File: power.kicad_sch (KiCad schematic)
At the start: 27 parts, among them IC1 SiC437BED-T1-GE3, J4 Barrel_Jack_Switch, Q1 PXP012-30QLJ, Q2 PXP012-30QLJ, U2 LTC4412xS6

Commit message: update 2 everything is fixed
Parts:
- R4, R5: footprint Resistor_SMD:R_2010_5025Metric_Pad1.40x2.65mm_HandSolder -> Resistor_SMD:R_0402_1005Metric
- R6: footprint Resistor_SMD:R_0603_1608Metric_Pad0.98x0.95mm_HandSolder -> Resistor_SMD:R_0402_1005Metric
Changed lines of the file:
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@@
 			)
 		)
-		(property "Footprint" "Resistor_SMD:R_0603_1608Metric_Pad0.98x0.95mm_HandSolder"
+		(property "Footprint" "Resistor_SMD:R_0402_1005Metric"
 			(at 234.95 59.69 0)
 			(effects
@@
 			)
 		)
-		(property "Footprint" "Resistor_SMD:R_2010_5025Metric_Pad1.40x2.65mm_HandSolder"
+		(property "Footprint" "Resistor_SMD:R_0402_1005Metric"
 			(at 201.93 50.8 0)
 			(effects
@@
 			)
 		)
-		(property "Footprint" "Resistor_SMD:R_2010_5025Metric_Pad1.40x2.65mm_HandSolder"
+		(property "Footprint" "Resistor_SMD:R_0402_1005Metric"
 			(at 201.93 48.26 0)
 			(effects

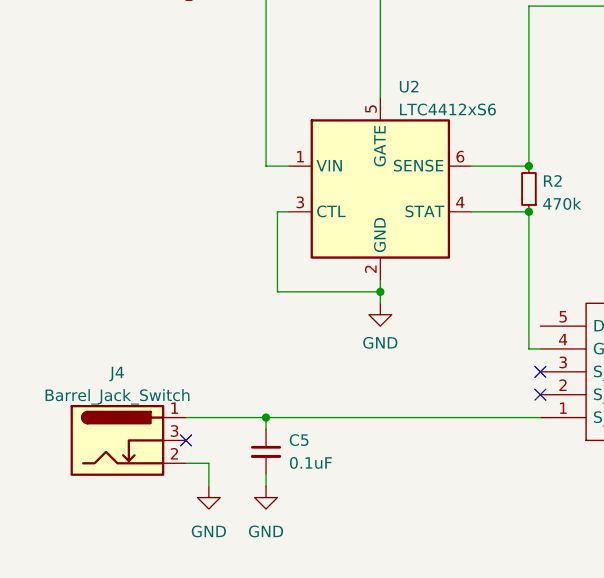
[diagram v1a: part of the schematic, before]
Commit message: ideal diode update to be checked
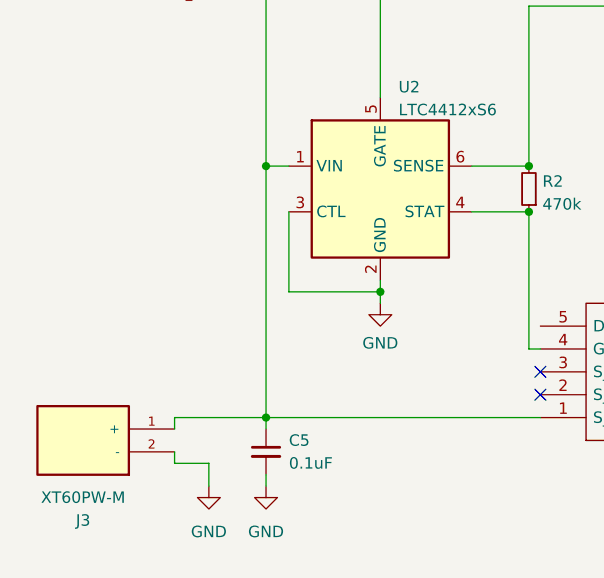
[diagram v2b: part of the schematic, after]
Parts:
- removed J4: Barrel_Jack_Switch, Connector_BarrelJack:BarrelJack_Wuerth_6941xx301002, symbol Connector:Barrel_Jack_Switch
- added J3: XT60PW-M, iclr:AMASS_XT60PW-M, symbol ICLR:XT60PW-M
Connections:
- net +BATTV: now also C5.1, Q2.1 (S_1), J3.1 (+)
- net GND: now also J3.2 (-)
- no-connect marks 17 -> 16
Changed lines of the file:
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@@
 	)
 	(junction
+		(at 44.45 58.42)
+		(diameter 0)
+		(color 0 0 0 0)
+	)
+	(junction
 		(at 196.85 90.17)
 		(diameter 0)
@@
 	)
 	(no_connect
-		(at 35.56 88.9)
-	)
-	(no_connect
 		(at 156.21 60.96)
 	)
@@
 	(wire
 		(pts
+			(xy 44.45 58.42) (xy 44.45 86.36)
+		)
+		(stroke
+			(width 0)
+			(type default)
+		)
+	)
+	(wire
+		(pts
 			(xy 67.31 63.5) (xy 73.66 63.5)
 		)
@@
 	(wire
 		(pts
-			(xy 57.15 71.12) (xy 57.15 72.39)
+			(xy 34.29 87.63) (xy 34.29 86.36)
 		)
 		(stroke
@@
 	(wire
 		(pts
-			(xy 191.77 66.04) (xy 194.31 66.04)
+			(xy 57.15 71.12) (xy 57.15 72.39)
 		)
 		(stroke
@@
 	(wire
 		(pts
-			(xy 217.17 85.09) (xy 217.17 83.82)
+			(xy 191.77 66.04) (xy 194.31 66.04)
 		)
 		(stroke
@@
 	(wire
 		(pts
-			(xy 46.99 63.5) (xy 45.72 63.5)
+			(xy 34.29 90.17) (xy 34.29 91.44)
 		)
 		(stroke
@@
 	(wire
 		(pts
-			(xy 101.6 81.28) (xy 101.6 62.23)
+			(xy 217.17 85.09) (xy 217.17 83.82)
 		)
 		(stroke
@@
 	(wire
 		(pts
-			(xy 148.59 50.8) (xy 148.59 53.34)
+			(xy 101.6 81.28) (xy 101.6 62.23)
 		)
 		(stroke
@@
 	(wire
 		(pts
-			(xy 35.56 91.44) (xy 38.1 91.44)
+			(xy 148.59 50.8) (xy 148.59 53.34)
 		)
 		(stroke
@@
 	(wire
 		(pts
-			(xy 45.72 63.5) (xy 45.72 72.39)
+			(xy 46.99 63.5) (xy 46.99 72.39)
 		)
 		(stroke
@@
 	(wire
 		(pts
-			(xy 44.45 58.42) (xy 46.99 58.42)
+			(xy 187.96 83.82) (xy 196.85 83.82)
 		)
 		(stroke
@@
 	(wire
 		(pts
-			(xy 187.96 83.82) (xy 196.85 83.82)
+			(xy 241.3 68.58) (xy 241.3 59.69)
 		)
 		(stroke
@@
 	(wire
 		(pts
-			(xy 241.3 68.58) (xy 241.3 59.69)
+			(xy 185.42 90.17) (xy 196.85 90.17)
 		)
 		(stroke
@@
 	(wire
 		(pts
-			(xy 185.42 90.17) (xy 196.85 90.17)
+			(xy 147.32 35.56) (xy 147.32 38.1)
 		)
 		(stroke
@@
 	(wire
 		(pts
-			(xy 147.32 35.56) (xy 147.32 38.1)
+			(xy 143.51 63.5) (xy 143.51 73.66)
 		)
 		(stroke
@@
 	(wire
 		(pts
-			(xy 143.51 63.5) (xy 143.51 73.66)
+			(xy 67.31 58.42) (xy 73.66 58.42)
 		)
 		(stroke
@@
 	(wire
 		(pts
-			(xy 67.31 58.42) (xy 73.66 58.42)
+			(xy 34.29 86.36) (xy 44.45 86.36)
 		)
 		(stroke
@@
 	(wire
 		(pts
+			(xy 44.45 58.42) (xy 46.99 58.42)
+		)
+		(stroke
+			(width 0)
+			(type default)
+		)
+	)
+	(wire
+		(pts
 			(xy 87.63 40.64) (xy 101.6 40.64)
 		)
@@
 	(wire
 		(pts
-			(xy 45.72 72.39) (xy 57.15 72.39)
+			(xy 46.99 72.39) (xy 57.15 72.39)
 		)
 		(stroke
@@
 	(wire
 		(pts
-			(xy 35.56 86.36) (xy 44.45 86.36)
-		)
-		(stroke
-			(width 0)
-			(type default)
-		)
-	)
-	(wire
-		(pts
 			(xy 143.51 45.72) (xy 143.51 63.5)
 		)
@@
 	(wire
 		(pts
+			(xy 34.29 91.44) (xy 38.1 91.44)
+		)
+		(stroke
+			(width 0)
+			(type default)
+		)
+	)
+	(wire
+		(pts
 			(xy 132.08 50.8) (xy 132.08 38.1)
 		)
@@
 	)
 	(symbol
-		(lib_id "Connector:Barrel_Jack_Switch")
-		(at 27.94 88.9 0)
-		(unit 1)
-		(exclude_from_sim no)
-		(in_bom yes)
-		(on_board yes)
-		(dnp no)
-		(property "Reference" "J4"
-			(at 27.94 81.3902 0)
-			(effects
-				(font
-					(size 1.27 1.27)
-				)
-			)
-		)
-		(property "Value" "Barrel_Jack_Switch"
-			(at 27.94 83.9271 0)
-			(effects
-				(font
-					(size 1.27 1.27)
-				)
-			)
-		)
-		(property "Footprint" "Connector_BarrelJack:BarrelJack_Wuerth_6941xx301002"
-			(at 29.21 89.916 0)
-			(effects
-				(font
-					(size 1.27 1.27)
-				)
-				(hide yes)
-			)
-		)
-		(property "Datasheet" "~"
-			(at 29.21 89.916 0)
-			(effects
-				(font
-					(size 1.27 1.27)
-				)
-				(hide yes)
-			)
-		)
-		(property "Description" ""
-			(at 27.94 88.9 0)
-			(effects
-				(font
-					(size 1.27 1.27)
-				)
-				(hide yes)
-			)
-		)
-		(pin "1"
-		)
-		(pin "2"
-		)
-		(pin "3"
-		)
-		(instances
-			(project "BetetrDom"
-				(path "/3d73b00f-865e-402b-88ef-ae22e0a8ba36/837d0d5a-cb41-4001-b9fc-855d4a9018ff"
-					(reference "J4")
-					(unit 1)
-				)
-			)
-		)
-	)
-	(symbol
 		(lib_id "power:VCC")
 		(at 110.49 58.42 0)
@@
 					(unit 1)
 				)
+			)
+		)
+	)
+	(symbol
+		(lib_id "ICLR:XT60PW-M")
+		(at 24.13 90.17 0)
+		(mirror y)
+		(unit 1)
+		(exclude_from_sim no)
+		(in_bom yes)
+		(on_board yes)
+		(dnp no)
+		(property "Reference" "J3"
+			(at 24.13 97.79 0)
+			(effects
+				(font
+					(size 1.27 1.27)
+				)
+			)
+		)
+		(property "Value" "XT60PW-M"
+			(at 24.13 95.25 0)
+			(effects
+				(font
+					(size 1.27 1.27)
+				)
+			)
+		)
+		(property "Footprint" "iclr:AMASS_XT60PW-M"
+			(at 24.13 90.17 0)
+			(effects
+				(font
+					(size 1.27 1.27)
+				)
+				(justify bottom)
+				(hide yes)
+			)
+		)
+		(property "Datasheet" ""
+			(at 24.13 90.17 0)
+			(effects
+				(font
+					(size 1.27 1.27)
+				)
+				(hide yes)
+			)
+		)
+		(property "Description" ""
+			(at 24.13 90.17 0)
+			(effects
+				(font
+					(size 1.27 1.27)
+				)
+				(hide yes)
+			)
+		)
+		(property "STANDARD" "Manufacturer recommendations"
+			(at 24.13 90.17 0)
+			(effects
+				(font
+					(size 1.27 1.27)
+				)
+				(justify bottom)
+				(hide yes)
+			)
+		)
+		(property "MANUFACTURER" "AMASS"
+			(at 24.13 90.17 0)
+			(effects
+				(font
+					(size 1.27 1.27)
+				)
+				(justify bottom)
+				(hide yes)
+			)
+		)
+		(property "PARTREV" "V1.2"
+			(at 24.13 90.17 0)
+			(effects
+				(font
+					(size 1.27 1.27)
+				)
+				(justify bottom)
+				(hide yes)
+			)
+		)
+		(property "MAXIMUM_PACKAGE_HEIGHT" "8.4 mm"
+			(at 24.13 90.17 0)
+			(effects
+				(font
+					(size 1.27 1.27)
+				)
+				(justify bottom)
+				(hide yes)
+			)
+		)
+		(pin "1"
+		)
+		(pin "2"
+		)
+		(instances
+			(project "BetetrDom"
+				(path "/3d73b00f-865e-402b-88ef-ae22e0a8ba36/837d0d5a-cb41-4001-b9fc-855d4a9018ff"
+					(reference "J3")
+					(unit 1)
+				)
